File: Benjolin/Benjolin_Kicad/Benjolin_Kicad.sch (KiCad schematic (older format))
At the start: 109 parts, among them U1 TL074, U2 TL072, U3 TL074, U4 TL074, U5 SSI2164, U6 4021

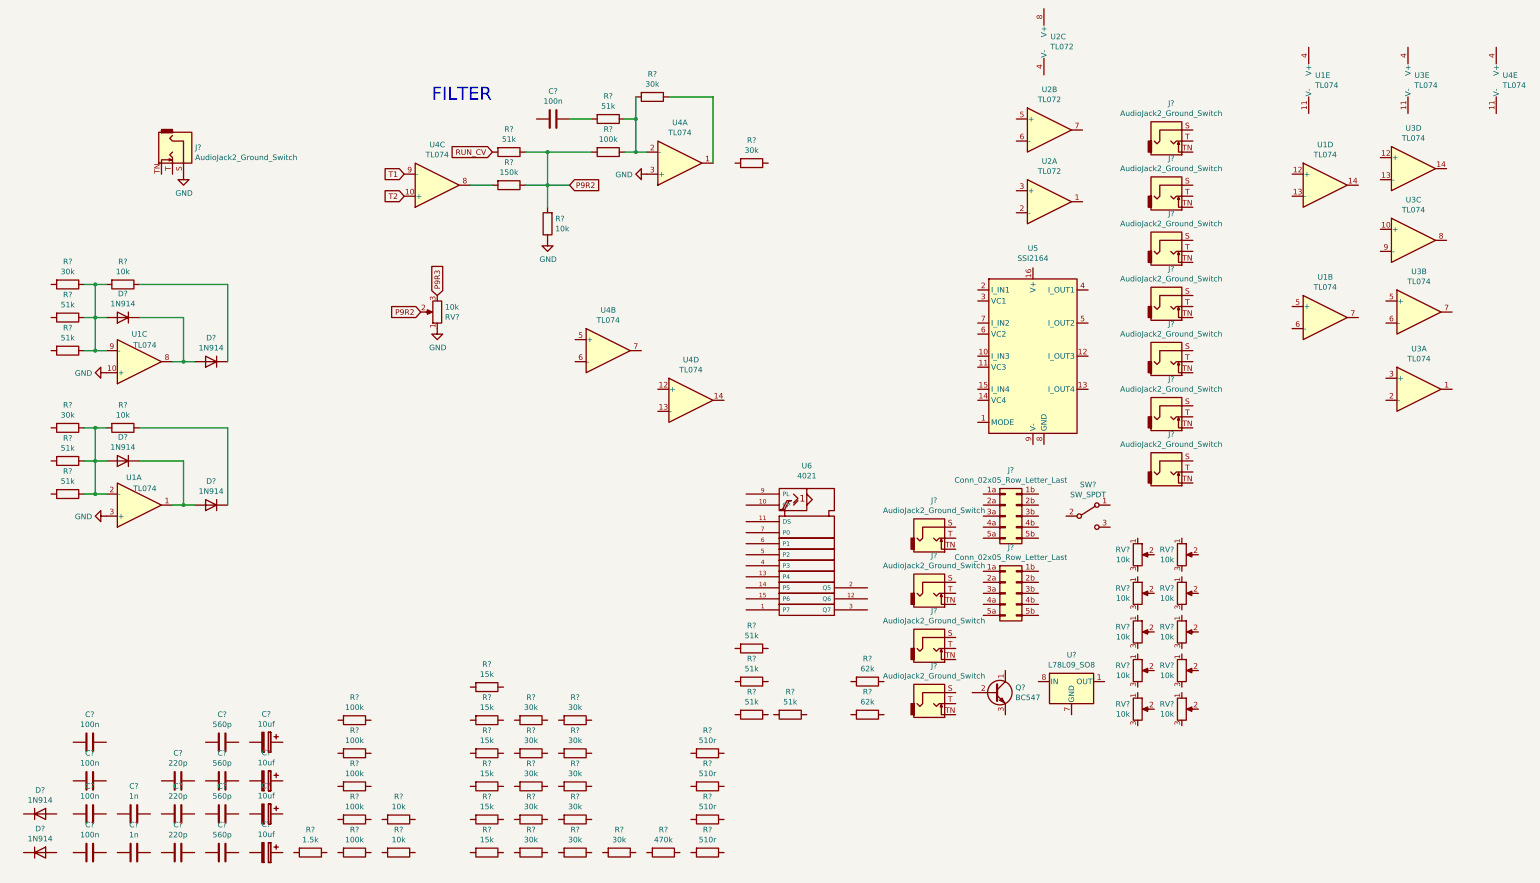
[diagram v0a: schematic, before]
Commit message: Nearly done with schematic
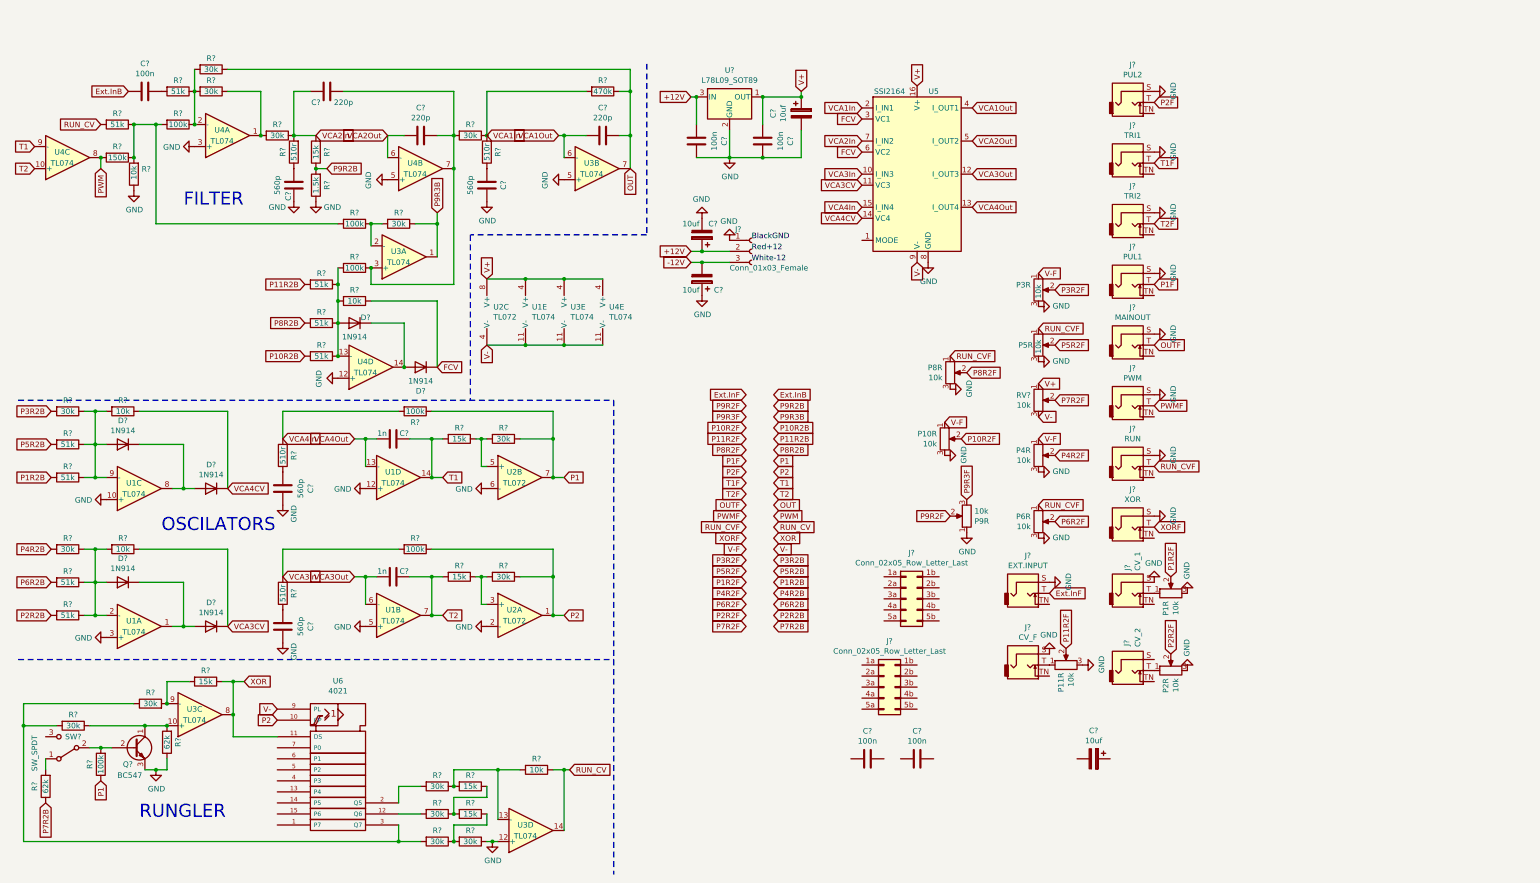
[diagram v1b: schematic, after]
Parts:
- removed R?: 51k, symbol Device:R
- removed U?: L78L09_SO8, Package_SO:SOIC-8_3.9x4.9mm_P1.27mm, symbol Regulator_Linear:L78L09_SO8
- added J?: Conn_01x03_Female, symbol Connector:Conn_01x03_Female
- added U?: L78L09_SOT89, Package_TO_SOT_SMD:SOT-89-3, symbol Regulator_Linear:L78L09_SOT89
- J?: value AudioJack2_Ground_Switch -> XOR
- J?: value AudioJack2_Ground_Switch -> RUN
- J?: value AudioJack2_Ground_Switch -> PWM
- J?: value AudioJack2_Ground_Switch -> MAINOUT
- J?: value AudioJack2_Ground_Switch -> CV_1
- J?: value AudioJack2_Ground_Switch -> CV_2
- J?: value AudioJack2_Ground_Switch -> PUL1
- J?: value AudioJack2_Ground_Switch -> TRI2
- J?: value AudioJack2_Ground_Switch -> TRI1
- J?: value AudioJack2_Ground_Switch -> PUL2
- J?: value AudioJack2_Ground_Switch -> CV_F
- J?: value AudioJack2_Ground_Switch -> EXT.INPUT
- gave numbers to parts that had none: 10
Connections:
- net GND: now also C?.1, C?.1, C?.1, C?.1, C?.1, C?.1, C?.1, C?.2, C?.2, J?.S, J?.S, J?.S, J?.S, J?.S, J?.S, J?.S, J?.S, J?.S, J?.S, P10R.3, P11R.3, P1R.3, P2R.3, P3R.3, P4R.3, P5R.3, P6R.3, P8R.3, Q?.3 (E), R?.1, R?.1, R?.1, U1.12 (+), U1.5 (+), U2.2 (-), U2.6 (-), U3.12 (+), U3.5 (+), U4.12 (+), U4.5 (+), U5.8 (GND), J?.1 (Pin_1), U?.2 (GND)
- net RUN_CV: now also R?.1, U3.14
- net T1: now also C?.1, R?.2, U1.14
- net T2: now also C?.1, R?.2, U1.7
- net FCV: now reaches D?.1 (K)
- net FCV: now also R?.1, U5.3 (VC1), U5.6 (VC2)
- net at D?.2 (A): now also D?.1 (K), U4.14
- net at D?.2 (A): now also R?.1, R?.1, R?.1, R?.2, R?.2, U4.13 (-)
- net VCA3CV: now reaches D?.1 (K), R?.1
- net VCA3CV: now also U5.11 (VC3)
- net VCA4CV: now reaches D?.1 (K), R?.1
- net VCA4CV: now also U5.14 (VC4)
- net V+: now reaches C?.2
- net V+: now also C?.1, RV?.1, U1.4 (V+), U2.8 (V+), U3.4 (V+), U4.4 (V+), U5.16 (V+), U?.1 (OUT)
- net +12V: now reaches C?.2
- net +12V: now also C?.1, J?.2 (Pin_2), U?.3 (IN)
- net Ext.InB: now reaches C?.2
- net VCA3Out: now reaches C?.2
- net VCA3Out: now also U1.6 (-), U5.12 (I_OUT3)
- net VCA4Out: now reaches C?.2
- net VCA4Out: now also U1.13 (-), U5.13 (I_OUT4)
- net OUT: now reaches C?.1
- net OUT: now also R?.1, R?.1, U3.7
- net VCA1Out: now reaches C?.2
- net VCA1Out: now also U3.6 (-), U5.4 (I_OUT1)
- net at C?.1: now also C?.1, R?.1, R?.2, U3.3 (+), U4.7
- net VCA2Out: now reaches C?.2
- net VCA2Out: now also U4.6 (-), U5.5 (I_OUT2)
- net VCA2In: now reaches C?.2
- net VCA2In: now also R?.1, R?.2, R?.2, U5.7 (I_IN2)
- net at C?.2: now also R?.1 (x4)
- net -12V: now reaches C?.2
- net -12V: now also J?.3 (Pin_3)
- net P9R2B: now reaches R?.2
- net P9R2B: now also R?.1
- net P1: now reaches R?.1
- net P1: now also R?.1, R?.1, U2.7
- net at R?.2: now also Q?.2 (B), SW?.2 (B)
- net P2: now reaches R?.1
- net P2: now also R?.1, U2.1, U6.10 (CP)
- net VCA3In: now reaches R?.2
- net VCA3In: now also R?.2, U5.10 (I_IN3)
- net VCA4In: now reaches R?.2
- net VCA4In: now also R?.2, U5.15 (I_IN4)
- net at R?.1: now also R?.2, U3.2 (-)
- net at R?.2: now also R?.1, R?.1, R?.2, R?.2
- net at R?.1, R?.1, R?.2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: now also R?.2
- net at R?.2: now also R?.1, R?.2, U3.13 (-)
- net PWM: now reaches R?.2, U4.8
- net XOR: now reaches R?.1
- net XOR: now also U3.8, U6.11 (DS)
- net at R?.2: now also R?.2, U3.9 (-)
- net at R?.1: now also R?.2, U2.3 (+)
- net at R?.1: now also R?.2, U2.5 (+)
- net at R?.1: now also R?.1, R?.2
- net at R?.2: now also R?.1, R?.1
- net at R?.1: now also Q?.1 (C), R?.2, U3.10 (+)
- net at R?.2: now also R?.1, R?.2, U6.3 (Q7)
- net at R?.2: now also U6.12 (Q6)
- net at R?.2: now also U6.2 (Q5)
- net at R?.2: now also R?.1, U4.1
- net P4R2B: now reaches R?.2
- net P3R2B: now reaches R?.2
- net VCA1In: now reaches R?.1
- net VCA1In: now also R?.2, R?.2, U5.2 (I_IN1)
- net P9R3B: now reaches R?.1
- net P9R3B: now also U3.1
- net P8R2B: now reaches R?.2
- net P10R2B: now reaches R?.2
- net P1R2B: now reaches R?.2
- net P5R2B: now reaches R?.2
- net P11R2B: now reaches R?.2
- net P6R2B: now reaches R?.2
- net P7R2B: now reaches R?.1
- net at R?.2: now also SW?.1 (A)
- net P7R2F: now reaches RV?.2
- net V-: now reaches RV?.3
- net V-: now also U1.11 (V-), U2.4 (V-), U3.11 (V-), U4.11 (V-), U5.9 (V-), U6.9 (PL)
- net at P2R.1: now also J?.T
- net P2R2F: now reaches P2R.2
- net at P11R.1: now also J?.T
- net P11R2F: now reaches P11R.2
- net V-F: now reaches P10R.1
- net V-F: now also P3R.1, P4R.1
- net P10R2F: now reaches P10R.2
- net RUN_CVF: now reaches P8R.1
- net RUN_CVF: now also J?.T, P5R.1, P6R.1
- net P8R2F: now reaches P8R.2
- net P6R2F: now reaches P6R.2
- net P4R2F: now reaches P4R.2
- net at P1R.1: now also J?.T
- net P1R2F: now reaches P1R.2
- net P5R2F: now reaches P5R.2
- net P3R2F: now reaches P3R.2
- net XORF: now reaches J?.T
- net PWMF: now reaches J?.T
- net OUTF: now reaches J?.T
- net P1F: now reaches J?.T
- net T2F: now reaches J?.T
- net T1F: now reaches J?.T
- net P2F: now reaches J?.T
- net Ext.InF: now reaches J?.T
- net P2R2B: now reaches R?.2
- removed net P9R2: P9R.2, R?.1, R?.1, R?.2, R?.2
- net P9R3 renamed P9R3F
- new net P9R2F: P9R.2
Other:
- note added: "OSCILATORS"
- note added: "RUNGLER"
- moved on the sheet: C?, D?, J?, P10R, P11R, P1R, P2R, P3R, P4R, P5R, P6R, P8R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
